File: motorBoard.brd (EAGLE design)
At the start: 127 x 76.3 mm, 74 parts

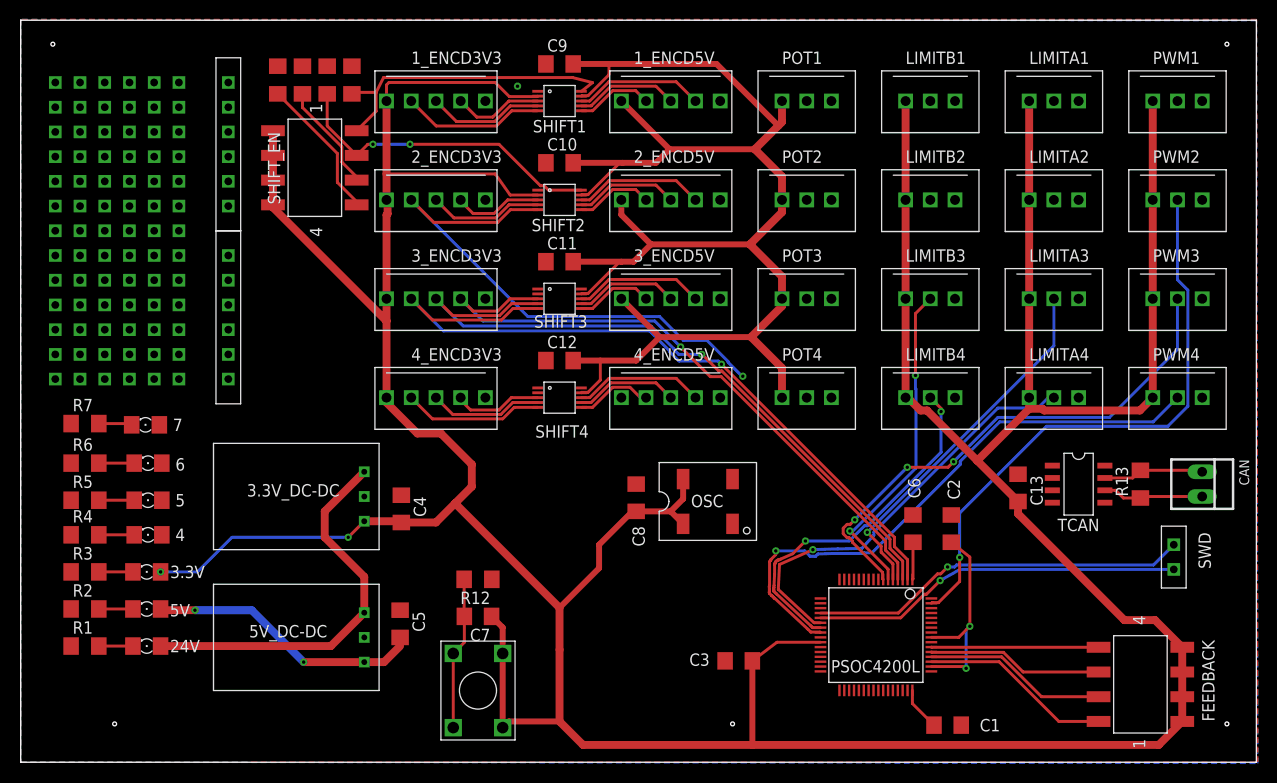
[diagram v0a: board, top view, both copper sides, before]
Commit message: Finished Board
Ready for Review
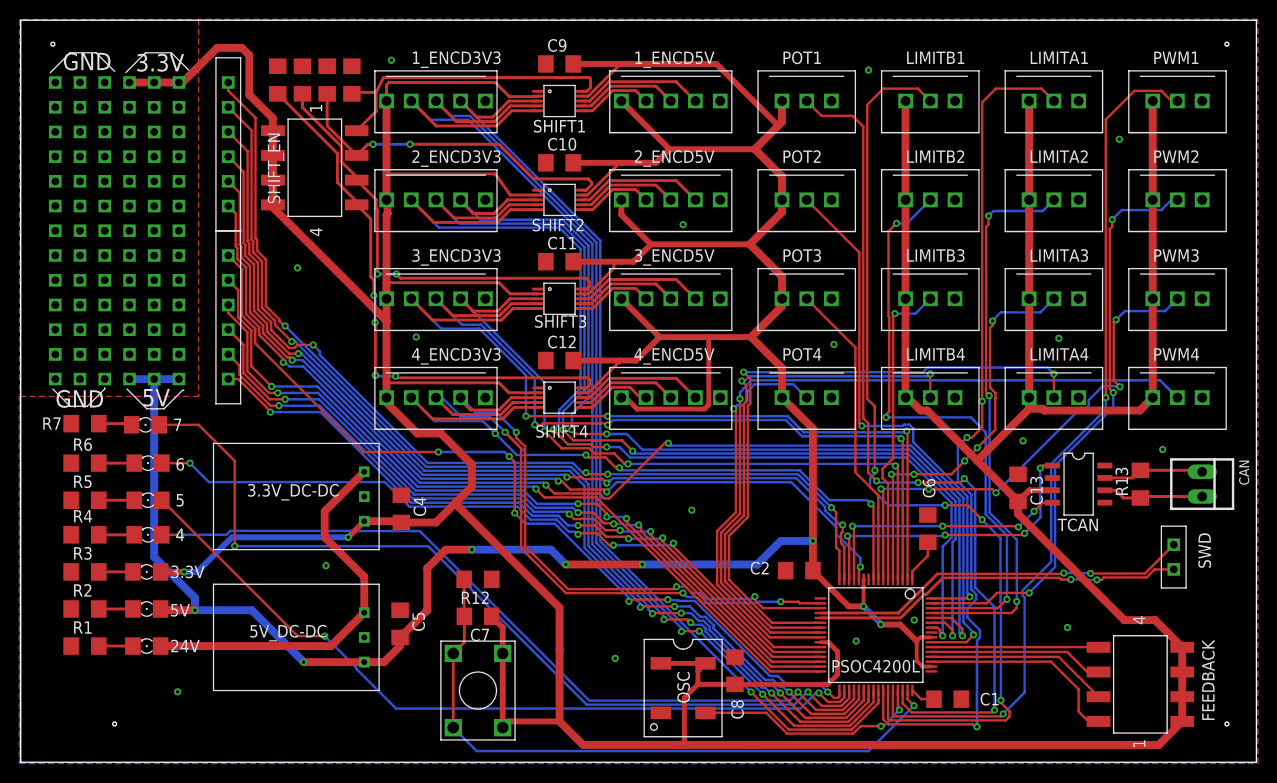
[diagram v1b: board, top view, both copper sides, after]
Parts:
- removed C3: 0.1uF, eagle-ltspice:C1206
- moved C8 20.5 mm to (73.4, 9.40)
- moved OSC 19.3 mm to (68.1, 7.62), turned to 270 degrees
- moved C2 16.2 mm to (80.0, 19.7), turned to 0 degrees
- moved C1 2.67 mm to (95.2, 6.48)
- moved C6 1.52 mm to (93.2, 24.0)
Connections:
- net +3V3: now also U$1.73, U$1.74, U$1.75; no longer C3.2
- net +5V: now also U$1.1, U$1.2, U$1.3
- net GNDA: now also U$1.4, U$1.5, U$1.6, U$1.76, U$1.77, U$1.78; no longer C3.1
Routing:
- net BASIC_HEADER2-1: track 0.00 -> 117.9 mm, vias 0 -> 4
- net +5V: track 208.6 -> 326.3 mm, vias 4 -> 8
- net BASIC_HEADER2-6: track 0.00 -> 109.6 mm, vias 0 -> 4
- net BASIC_HEADER2-5: track 0.00 -> 106.7 mm, vias 0 -> 4
- net MOTOR1LIMB: track 0.00 -> 97.5 mm, vias 0 -> 4
- net MOTOR2A2: track 11.8 -> 109.1 mm, vias 0 -> 3
- net MOTOR2A1: track 9.14 -> 105.2 mm, vias 0 -> 3
- net BASIC_HEADER2-4: track 0.00 -> 95.5 mm, vias 0 -> 4
- net MOTOR1A3: track 14.7 -> 108.8 mm, vias 0 -> 3
- net BASIC_HEADER2-3: track 0.00 -> 93.4 mm, vias 0 -> 4
- net MOTOR1A2: track 12.0 -> 104.1 mm, vias 0 -> 3
- net BASIC_HEADER2-2: track 0.00 -> 91.6 mm, vias 0 -> 4
- net MOTOR1A1: track 9.28 -> 99.5 mm, vias 0 -> 1
- net LED7: track 0.00 -> 90.2 mm, vias 0 -> 2
- net MOTOR1POT: track 0.00 -> 89.5 mm, vias 0 -> 4
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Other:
- board text added: "3.3V"
- board text added: "5V"
- board text added: "GND"

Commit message: Revert "Finished Board"
This reverts commit 761fd842cb1d32e6d861dcd06b5bacfd84886b14.
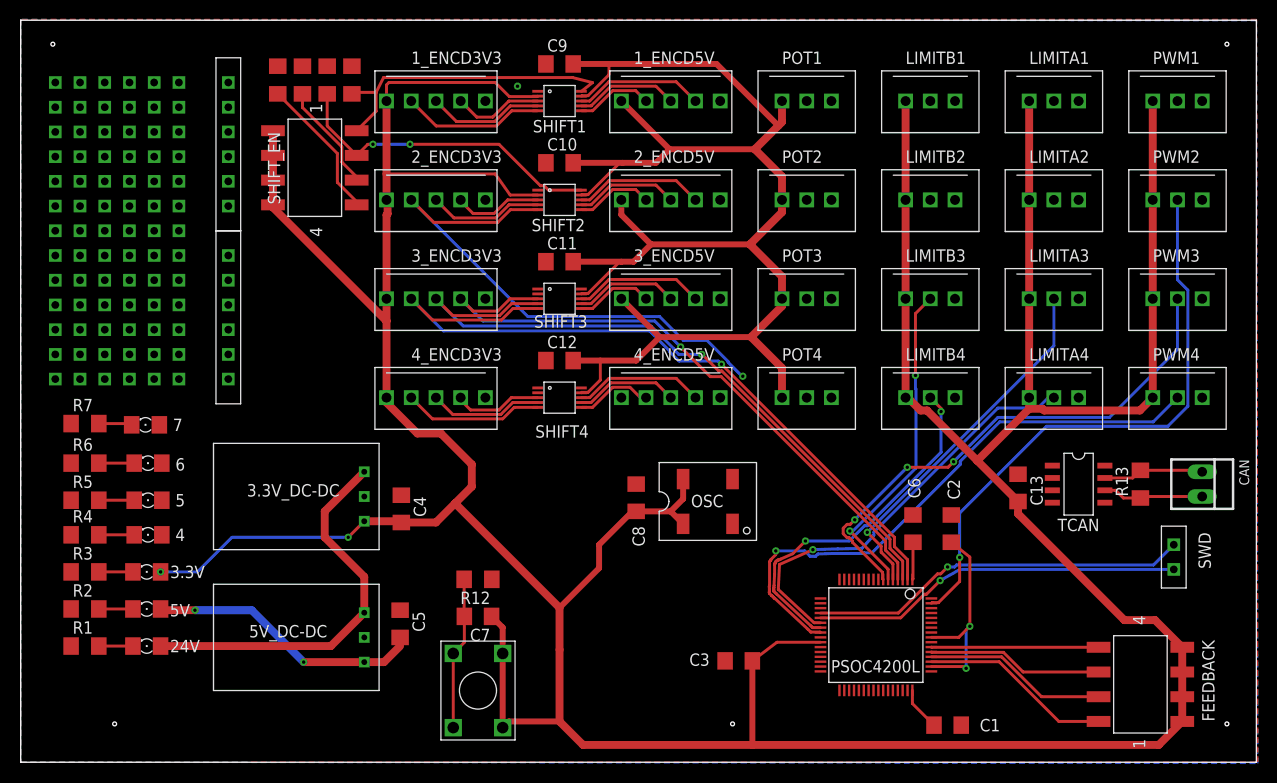
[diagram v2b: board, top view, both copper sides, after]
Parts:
- added C3: 0.1uF, eagle-ltspice:C1206
- moved C8 20.5 mm to (63.2, 27.2)
- moved OSC 19.3 mm to (70.6, 26.8), turned to 0 degrees
- moved C2 16.2 mm to (95.6, 24.0), turned to 270 degrees
- moved C1 2.67 mm to (95.2, 3.81)
- moved C6 1.52 mm to (91.7, 24.0)
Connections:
- net +3V3: now also C3.2; no longer U$1.73, U$1.74, U$1.75
- net +5V: no longer U$1.1, U$1.2, U$1.3
- net GNDA: now also C3.1; no longer U$1.4, U$1.5, U$1.6, U$1.76, U$1.77, U$1.78
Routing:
- net BASIC_HEADER2-1: track 117.9 -> 0.00 mm, vias 4 -> 0
- net +5V: track 326.3 -> 208.6 mm, vias 8 -> 4
- net BASIC_HEADER2-6: track 109.6 -> 0.00 mm, vias 4 -> 0
- net BASIC_HEADER2-5: track 106.7 -> 0.00 mm, vias 4 -> 0
- net MOTOR1LIMB: track 97.5 -> 0.00 mm, vias 4 -> 0
- net MOTOR2A2: track 109.1 -> 11.8 mm, vias 3 -> 0
- net MOTOR2A1: track 105.2 -> 9.14 mm, vias 3 -> 0
- net BASIC_HEADER2-4: track 95.5 -> 0.00 mm, vias 4 -> 0
- net MOTOR1A3: track 108.8 -> 14.7 mm, vias 3 -> 0
- net BASIC_HEADER2-3: track 93.4 -> 0.00 mm, vias 4 -> 0
- net MOTOR1A2: track 104.1 -> 12.0 mm, vias 3 -> 0
- net BASIC_HEADER2-2: track 91.6 -> 0.00 mm, vias 4 -> 0
- net MOTOR1A1: track 99.5 -> 9.28 mm, vias 1 -> 0
- net LED7: track 90.2 -> 0.00 mm, vias 2 -> 0
- net MOTOR1POT: track 89.5 -> 0.00 mm, vias 4 -> 0
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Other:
- board text removed: "3.3V"
- board text removed: "5V"
- board text removed: "GND"
